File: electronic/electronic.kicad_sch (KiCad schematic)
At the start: 22 parts, among them IC1 AS5600-ASOT, IC2 AS5600-ASOT, IC3 AS5600-ASOT, IC4 AS5600-ASOT, J2 BAT_AX, M1 ESC, M2 ESC, M3 ESC, M4 ESC, U1 ESP32-DEVKITC-V4, U13 SSD1306, U15 HC-SR04, U16 HC-SR04, U17 HC-SR04, U18 HC-SR04, U2 NEO-6M-GPS, U3 MPU-9250+BMP280, U4 TCA9548AMRGER

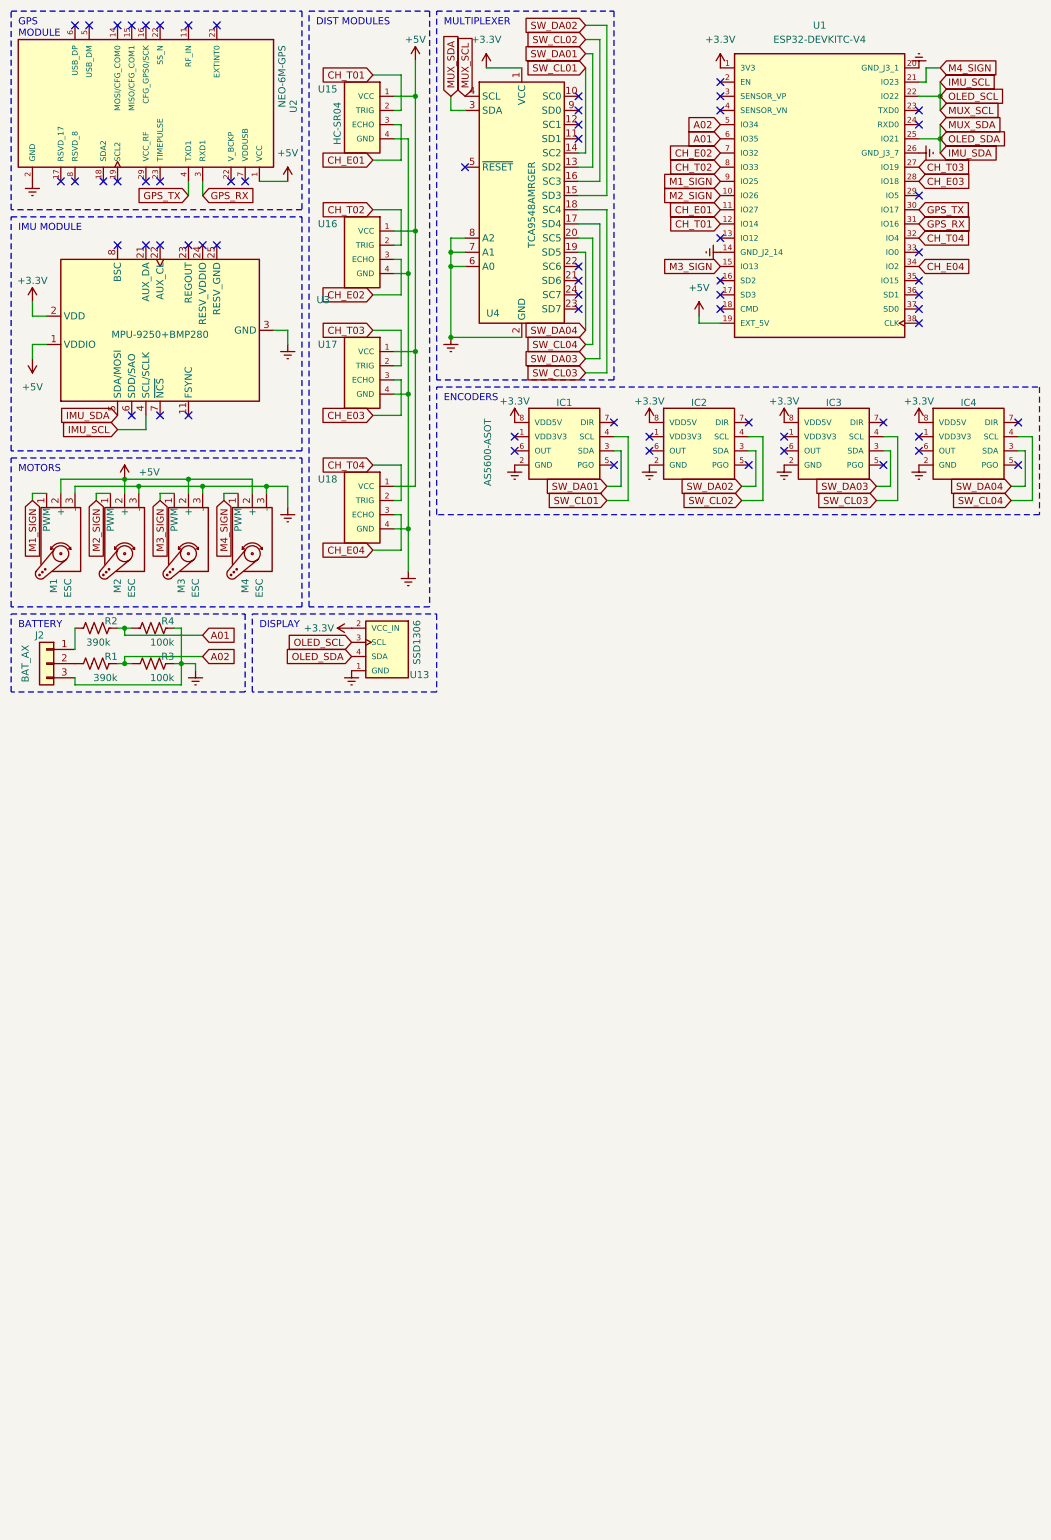
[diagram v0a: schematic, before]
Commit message: refactor: update PCB
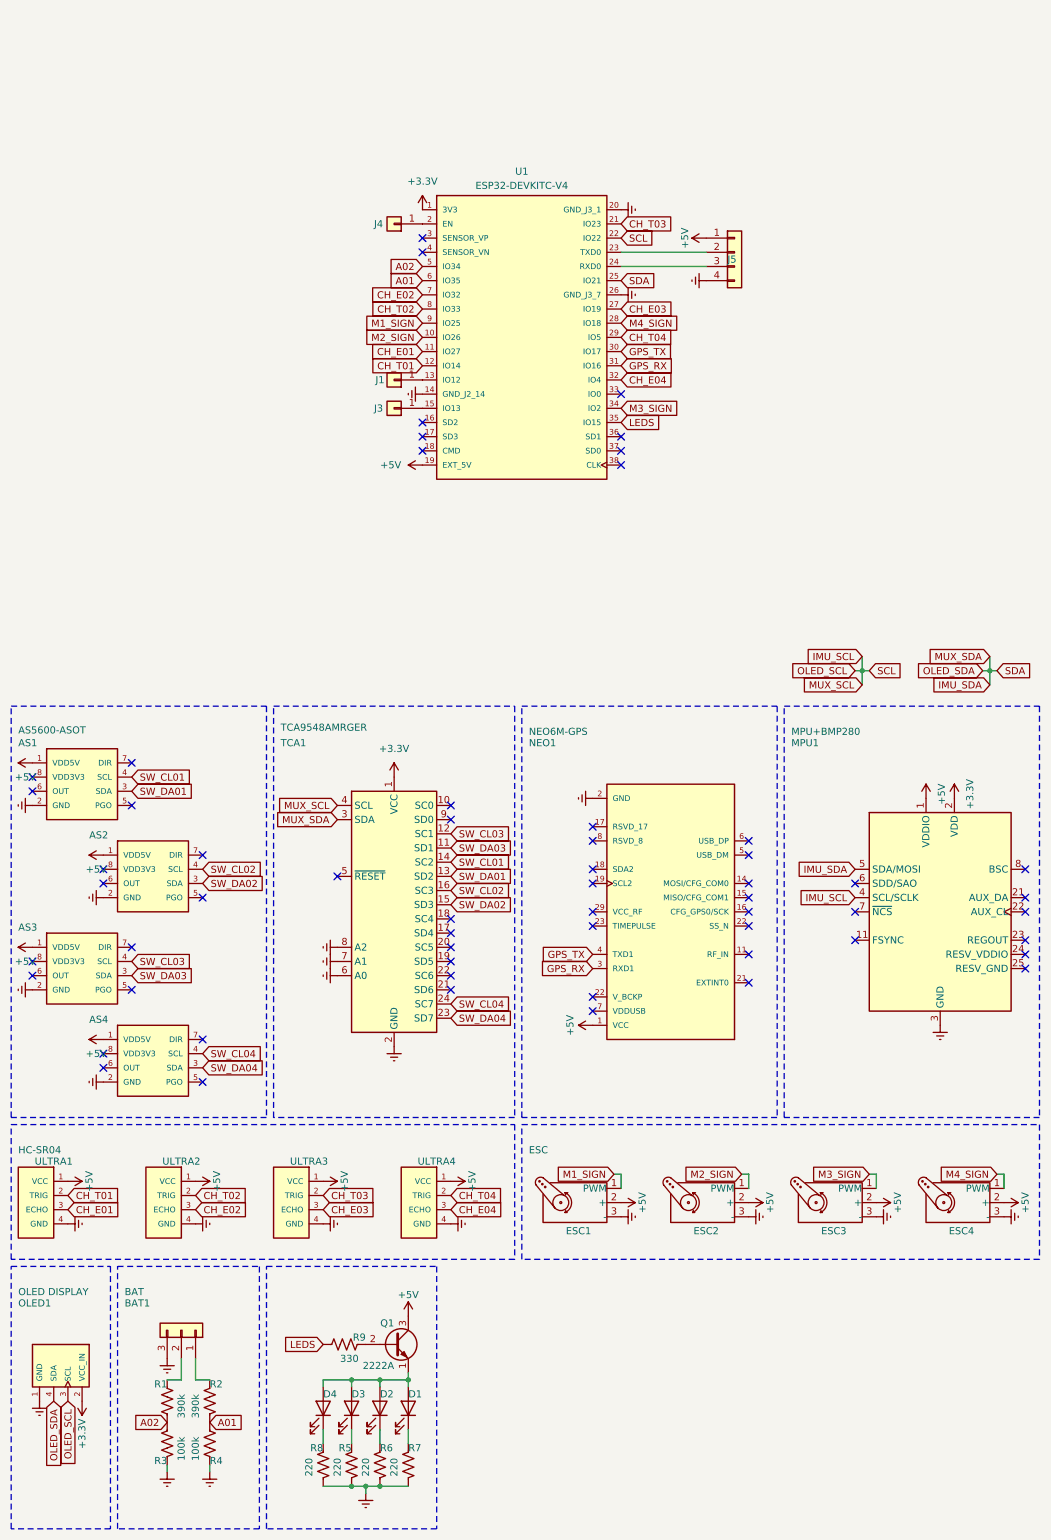
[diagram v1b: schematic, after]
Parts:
- removed M1, M2, M3, M4: ESC, Connector_PinSocket_2.54mm:PinSocket_1x03_P2.54mm_Horizontal, symbol Motor:Motor_Servo
- added D1, D2, D3, D4: LED, Connector_PinHeader_2.54mm:PinHeader_1x02_P2.54mm_Vertical, symbol Device:LED
- added ESC1: ESC, MYPCB:ESC1, symbol Motor:Motor_Servo
- added ESC2: ESC, MYPCB:ESC2, symbol Motor:Motor_Servo
- added ESC3: ESC, MYPCB:ESC3, symbol Motor:Motor_Servo
- added ESC4: ESC, MYPCB:ESC4, symbol Motor:Motor_Servo
- added J1, J3, J4: Conn_01x01, Connector_PinHeader_2.54mm:PinHeader_1x01_P2.54mm_Vertical, symbol Connector_Generic:Conn_01x01
- added J5: Conn_01x02, Connector_PinHeader_2.54mm:PinHeader_1x04_P2.54mm_Vertical, symbol Connector_Generic:Conn_01x04
- added Q1: 2222A, Package_TO_SOT_THT:TO-92_Inline, symbol Transistor_BJT:PN2222A
- added R5, R6, R7, R8: 220, Resistor_SMD:R_0805_2012Metric, symbol Device:R_US
- added R9: 330, Resistor_SMD:R_0805_2012Metric, symbol Device:R_US
- AS1: renamed from IC1; footprint AS5600-ASOT:SOIC127P600X175-8N -> Connector_PinSocket_2.54mm:PinSocket_1x04_P2.54mm_Horizontal
- AS2: renamed from IC2; footprint AS5600-ASOT:SOIC127P600X175-8N -> Connector_PinSocket_2.54mm:PinSocket_1x04_P2.54mm_Horizontal
- AS3: renamed from IC3; footprint AS5600-ASOT:SOIC127P600X175-8N -> Connector_PinSocket_2.54mm:PinSocket_1x04_P2.54mm_Horizontal
- AS4: renamed from IC4; footprint AS5600-ASOT:SOIC127P600X175-8N -> Connector_PinSocket_2.54mm:PinSocket_1x04_P2.54mm_Horizontal
- BAT1: renamed from J2; value BAT_AX -> BAT
- MPU1: renamed from U3; value MPU-9250+BMP280 -> MPU+BMP280
- NEO1: renamed from U2; value NEO-6M-GPS -> NEO6M-GPS
- OLED1: renamed from U13; value SSD1306 -> OLED DISPLAY
- ULTRA1: renamed from U15; footprint HC-SR04:XCVR_HC-SR04 -> Connector_PinSocket_2.54mm:PinSocket_1x04_P2.54mm_Horizontal
- ULTRA2: renamed from U16; footprint HC-SR04:XCVR_HC-SR04 -> Connector_PinSocket_2.54mm:PinSocket_1x04_P2.54mm_Horizontal
- ULTRA3: renamed from U17; footprint HC-SR04:XCVR_HC-SR04 -> Connector_PinSocket_2.54mm:PinSocket_1x04_P2.54mm_Horizontal
- ULTRA4: renamed from U18; footprint HC-SR04:XCVR_HC-SR04 -> Connector_PinSocket_2.54mm:PinSocket_1x04_P2.54mm_Horizontal
- renumbered U4 to TCA1
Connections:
- net +3.3V: no longer AS1.8 (VDD5V), AS2.8 (VDD5V), AS3.8 (VDD5V), AS4.8 (VDD5V)
- net +5V: now also AS1.1 (VDD5V), AS2.1 (VDD5V), AS3.1 (VDD5V), AS4.1 (VDD5V), ESC1.2 (+), ESC2.2 (+), ESC3.2 (+), ESC4.2 (+), J5.1 (Pin_1), Q1.3 (C)
- net A01: now also R2.1; no longer R2.2
- net A02: now also R1.1; no longer R1.2
- net CH_E03: now also U1.27 (IO19); no longer U1.28 (IO18)
- net CH_E04: now also U1.32 (IO4); no longer U1.34 (IO2)
- net CH_T03: now also U1.21 (IO23); no longer U1.27 (IO19)
- net CH_T04: now also U1.29 (IO5); no longer U1.32 (IO4)
- net Earth: now also ESC1.3 (-), ESC2.3 (-), ESC3.3 (-), ESC4.3 (-), J5.4 (Pin_4), R5.1, R6.1, R7.1, R8.1
- net M1_SIGN: now also ESC1.1 (PWM)
- net M2_SIGN: now also ESC2.1 (PWM)
- net M3_SIGN: now also U1.34 (IO2), ESC3.1 (PWM); no longer U1.15 (IO13)
- net M4_SIGN: now also U1.28 (IO18), ESC4.1 (PWM); no longer U1.21 (IO23)
- net SW_CL03: now also TCA1.12 (SC1); no longer TCA1.18 (SC4)
- net SW_CL04: now also TCA1.24 (SC7); no longer TCA1.20 (SC5)
- net SW_DA03: now also TCA1.11 (SD1); no longer TCA1.17 (SD4)
- net SW_DA04: now also TCA1.23 (SD7); no longer TCA1.19 (SD5)
- net at U1.13 (IO12): now also J1.1 (Pin_1)
- net at U1.2 (EN): now also J4.1 (Pin_1)
- net at U1.23 (TXD0): now also J5.2 (Pin_2)
- net at U1.24 (RXD0): now also J5.3 (Pin_3)
- net LEDS: now reaches U1.35 (IO15)
- net LEDS: now also R9.1
- net at BAT1.1 (Pin_1): now also R2.2; no longer R2.1
- net at BAT1.2 (Pin_2): now also R1.2; no longer R1.1
- new net: D4.1 (K), R8.2
- new net: D1.2 (A), D2.2 (A), D3.2 (A), D4.2 (A), Q1.1 (E)
- new net: Q1.2 (B), R9.2
- new net: D2.1 (K), R6.2
- new net: J3.1 (Pin_1), U1.15 (IO13)
- new net: D3.1 (K), R5.2
- new net: D1.1 (K), R7.2
- no-connect marks 65 -> 59
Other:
- note removed: "BATTERY"
- note removed: "DISPLAY"
- note removed: "DIST MODULES"
- note removed: "ENCODERS"
- note removed: "GPS MODULE"
- note removed: "IMU MODULE"
- note removed: "MOTORS"
- note removed: "MULTIPLEXER"
- title: Squematico de la plataforma -> MAIN
- moved on the sheet: AS1, AS2, AS3, AS4, BAT1, MPU1, NEO1, OLED1, R1, R2, R3, R4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
